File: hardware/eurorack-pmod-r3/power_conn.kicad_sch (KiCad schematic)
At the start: 23 parts, among them J1 CONN 2x5 P=2.54mm, J2 CONN 2x6 P=2.54mm, J3 Conn_01x14_Socket

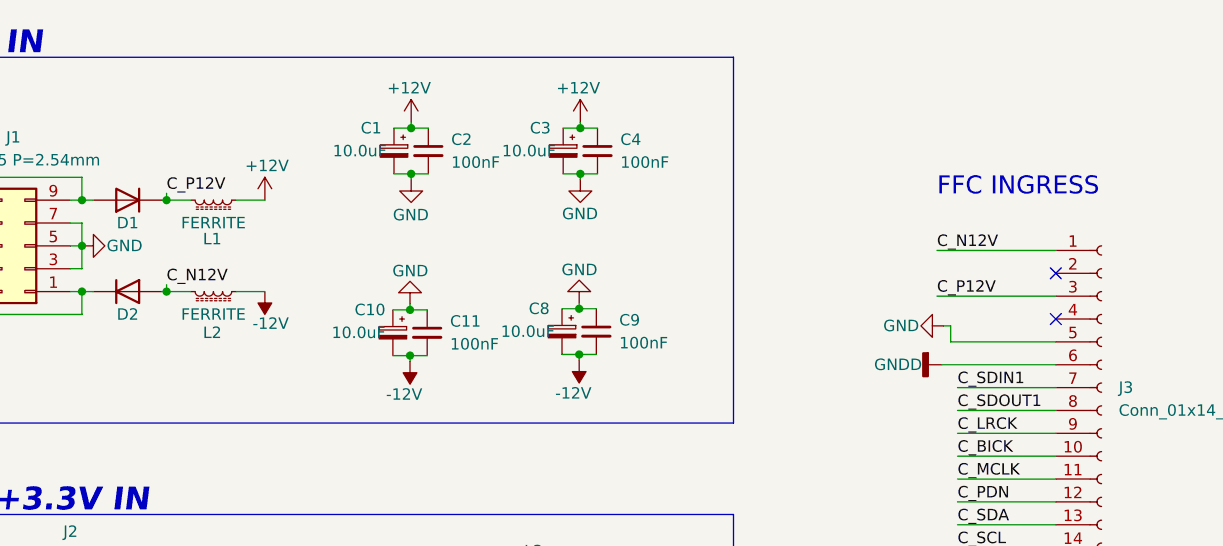
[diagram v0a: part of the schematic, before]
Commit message: Almost ready for layout
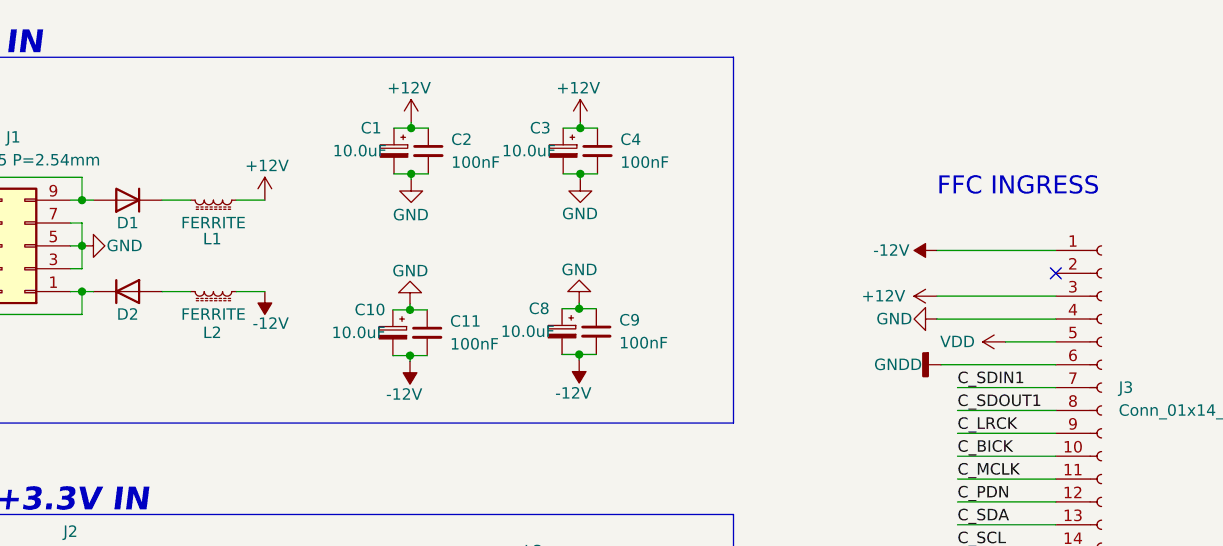
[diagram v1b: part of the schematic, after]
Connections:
- net +12V: now also J3.3 (Pin_3)
- net -12V: now also J3.1 (Pin_1)
- net GND: now also J3.4 (Pin_4); no longer J3.5 (Pin_5)
- net VDD: now also J3.5 (Pin_5)
- net C_N12V: no longer names the net of D2.2 (A), L2.2
- net C_N12V: no longer J3.1 (Pin_1)
- net C_P12V: no longer names the net of D1.1 (K), L1.2
- net C_P12V: no longer J3.3 (Pin_3)
- no-connect marks 2 -> 1
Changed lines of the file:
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@@
   (junction (at 45.72 88.9) (diameter 0) (color 0 0 0 0)
   )
-  (junction (at 50.038 43.18) (diameter 0) (color 0 0 0 0)
-  )
   (junction (at 96.012 30.099) (diameter 0) (color 0 0 0 0)
   )
@@
   (junction (at 25.4 38.1) (diameter 0) (color 0 0 0 0)
   )
-  (junction (at 50.038 33.02) (diameter 0) (color 0 0 0 0)
-  )
   (junction (at 77.089 50.292) (diameter 0) (color 0 0 0 0)
   )
@@
   (junction (at 102.235 94.615) (diameter 0) (color 0 0 0 0)
   )
-  (no_connect (at 148.844 46.228))
   (no_connect (at 148.844 41.148))
   (wire (pts (xy 75.184 45.212) (xy 77.089 45.212))
@@
     (stroke (width 0) (type default))
   )
-  (wire (pts (xy 50.038 43.18) (xy 52.705 43.18))
+  (wire (pts (xy 49.53 43.18) (xy 52.705 43.18))
     (stroke (width 0) (type default))
   )
@@
     (stroke (width 0) (type default))
   )
-  (wire (pts (xy 137.16 46.99) (xy 137.16 48.768))
-    (stroke (width 0) (type default))
-  )
   (wire (pts (xy 33.02 88.9) (xy 33.02 91.44))
     (stroke (width 0) (type default))
@@
     (stroke (width 0) (type default))
   )
-  (wire (pts (xy 49.53 33.02) (xy 50.038 33.02))
-    (stroke (width 0) (type default))
-  )
   (wire (pts (xy 136.144 51.308) (xy 148.844 51.308))
     (stroke (width 0) (type default))
@@
     (stroke (width 0) (type default))
   )
-  (wire (pts (xy 50.038 32.258) (xy 50.038 33.02))
-    (stroke (width 0) (type default))
-  )
   (wire (pts (xy 39.37 40.64) (xy 40.64 40.64))
     (stroke (width 0) (type default))
@@
     (stroke (width 0) (type default))
   )
-  (wire (pts (xy 50.038 42.418) (xy 50.038 43.18))
+  (wire (pts (xy 135.636 46.228) (xy 148.844 46.228))
     (stroke (width 0) (type default))
   )
@@
     (stroke (width 0) (type default))
   )
-  (wire (pts (xy 137.16 48.768) (xy 148.844 48.768))
-    (stroke (width 0) (type default))
-  )
   (wire (pts (xy 93.345 73.279) (xy 95.885 73.279))
     (stroke (width 0) (type default))
@@
     (stroke (width 0) (type default))
   )
-  (wire (pts (xy 50.038 33.02) (xy 52.705 33.02))
+  (wire (pts (xy 49.53 33.02) (xy 52.705 33.02))
     (stroke (width 0) (type default))
   )
@@
     (stroke (width 0) (type default))
   )
-  (wire (pts (xy 136.398 46.99) (xy 137.16 46.99))
-    (stroke (width 0) (type default))
-  )
   (wire (pts (xy 25.4 38.1) (xy 26.67 38.1))
     (stroke (width 0) (type default))
@@
     (stroke (width 0) (type default))
   )
-  (wire (pts (xy 49.53 43.18) (xy 50.038 43.18))
-    (stroke (width 0) (type default))
-  )
   (wire (pts (xy 40.64 35.56) (xy 40.64 38.1))
     (stroke (width 0) (type default))
@@
   )
   (polyline (pts (xy 113.03 128.905) (xy 16.51 128.905))
+    (stroke (width 0) (type default))
+  )
+  (wire (pts (xy 143.256 48.768) (xy 148.844 48.768))
     (stroke (width 0) (type default))
   )
@@
     (effects (font (size 1.27 1.27)) (justify left bottom))
   )
-  (label "C_N12V" (at 135.636 38.608 0) (fields_autoplaced)
-    (effects (font (size 1.27 1.27)) (justify left bottom))
-  )
   (label "C_SDOUT1" (at 24.13 78.74 0) (fields_autoplaced)
     (effects (font (size 1.27 1.27)) (justify left bottom))
@@
     (effects (font (size 1.27 1.27)) (justify left bottom))
   )
-  (label "C_P12V" (at 135.636 43.688 0) (fields_autoplaced)
-    (effects (font (size 1.27 1.27)) (justify left bottom))
-  )
   (label "C_SDIN1" (at 24.13 76.2 0) (fields_autoplaced)
     (effects (font (size 1.27 1.27)) (justify left bottom))
@@
     (effects (font (size 1.27 1.27)) (justify left bottom))
   )
-  (label "C_P12V" (at 50.038 32.258 0) (fields_autoplaced)
-    (effects (font (size 1.27 1.27)) (justify left bottom))
-  )
   (label "C_MCLK" (at 137.922 64.008 0) (fields_autoplaced)
     (effects (font (size 1.27 1.27)) (justify left bottom))
@@
   )
   (label "C_LRCK" (at 24.13 81.28 0) (fields_autoplaced)
-    (effects (font (size 1.27 1.27)) (justify left bottom))
-  )
-  (label "C_N12V" (at 50.038 42.418 0) (fields_autoplaced)
     (effects (font (size 1.27 1.27)) (justify left bottom))
   )
@@
     )
   )
-  (symbol (lib_id "power:GND") (at 136.398 46.99 270) (mirror x) (unit 1)
-    (in_bom yes) (on_board yes) (dnp no)
-    (property "Reference" "#PWR014" (at 130.048 46.99 0)
-      (effects (font (size 1.27 1.27)) hide)
-    )
-    (property "Value" "GND" (at 129.667 46.99 90)
+  (symbol (lib_id "power:GND") (at 135.636 46.228 270) (mirror x) (unit 1)
+    (in_bom yes) (on_board yes) (dnp no)
+    (property "Reference" "#PWR014" (at 129.286 46.228 0)
+      (effects (font (size 1.27 1.27)) hide)
+    )
+    (property "Value" "GND" (at 128.905 46.228 90)
       (effects (font (size 1.27 1.27)) (justify left))
     )
-    (property "Footprint" "" (at 136.398 46.99 0)
-      (effects (font (size 1.27 1.27)) hide)
-    )
-    (property "Datasheet" "" (at 136.398 46.99 0)
+    (property "Footprint" "" (at 135.636 46.228 0)
+      (effects (font (size 1.27 1.27)) hide)
+    )
+    (property "Datasheet" "" (at 135.636 46.228 0)
       (effects (font (size 1.27 1.27)) hide)
     )
@@
     )
   )
+  (symbol (lib_id "power:-12V") (at 135.636 38.608 90) (unit 1)
+    (in_bom yes) (on_board yes) (dnp no)
+    (property "Reference" "#PWR018" (at 133.096 38.608 0)
+      (effects (font (size 1.27 1.27)) hide)
+    )
+    (property "Value" "-12V" (at 132.588 38.608 90)
+      (effects (font (size 1.27 1.27)) (justify left))
+    )
+    (property "Footprint" "" (at 135.636 38.608 0)
+      (effects (font (size 1.27 1.27)) hide)
+    )
+    (property "Datasheet" "" (at 135.636 38.608 0)
+      (effects (font (size 1.27 1.27)) hide)
+    )
+    (pin "1")
+    (instances
+      (project "eurorack-pmod-pcb"
+        (path "/d1469efb-590b-4a61-a37b-5bbc286936ba"
+          (reference "#PWR018") (unit 1)
+        )
+        (path "/d1469efb-590b-4a61-a37b-5bbc286936ba/8bd0f3ad-78ad-46cf-a63b-58b9dbc835d8"
+          (reference "#PWR0115") (unit 1)
+        )
+      )
+    )
+  )
+  (symbol (lib_id "power:+12V") (at 135.636 43.688 90) (unit 1)
+    (in_bom yes) (on_board yes) (dnp no)
+    (property "Reference" "#PWR012" (at 139.446 43.688 0)
+      (effects (font (size 1.27 1.27)) hide)
+    )
+    (property "Value" "+12V" (at 127.254 43.688 90)
+      (effects (font (size 1.27 1.27)) (justify right))
+    )
+    (property "Footprint" "" (at 135.636 43.688 0)
+      (effects (font (size 1.27 1.27)) hide)
+    )
+    (property "Datasheet" "" (at 135.636 43.688 0)
+      (effects (font (size 1.27 1.27)) hide)
+    )
+    (pin "1")
+    (instances
+      (project "eurorack-pmod-pcb"
+        (path "/d1469efb-590b-4a61-a37b-5bbc286936ba"
+          (reference "#PWR012") (unit 1)
+        )
+        (path "/d1469efb-590b-4a61-a37b-5bbc286936ba/8bd0f3ad-78ad-46cf-a63b-58b9dbc835d8"
+          (reference "#PWR0114") (unit 1)
+        )
+      )
+    )
+  )
   (symbol (lib_id "Device:C_Polarized_Small") (at 93.98 113.665 0) (mirror y) (unit 1)
     (in_bom yes) (on_board yes) (dnp no)
@@
         )
       )
+    )
+  )
+  (symbol (lib_id "power:VDD") (at 143.256 48.768 90) (unit 1)
+    (in_bom yes) (on_board yes) (dnp no)
+    (property "Reference" "#PWR034" (at 147.066 48.768 0)
+      (effects (font (size 1.27 1.27)) hide)
+    )
+    (property "Value" "VDD" (at 137.922 48.768 90)
+      (effects (font (size 1.27 1.27)))
+    )
+    (property "Footprint" "" (at 143.256 48.768 0)
+      (effects (font (size 1.27 1.27)) hide)
+    )
+    (property "Datasheet" "" (at 143.256 48.768 0)
+      (effects (font (size 1.27 1.27)) hide)
+    )
+    (pin "1")
+    (instances
+      (project "eurorack-pmod-pcb"
+        (path "/d1469efb-590b-4a61-a37b-5bbc286936ba"
+          (reference "#PWR034") (unit 1)
+        )
+        (path "/d1469efb-590b-4a61-a37b-5bbc286936ba/8bd0f3ad-78ad-46cf-a63b-58b9dbc835d8"
+          (reference "#PWR0116") (unit 1)
+        )
+      )
